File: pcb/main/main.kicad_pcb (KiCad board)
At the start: 2 copper layers, 172.1 x 113 mm, 122 parts, among them J1 Conn_01x04, J10 JTAG, J2 USB_B, J3 Trackball_conn, J4 ROW0, J5 RJ45, J6 ROW1, J7 ROW2, J8 ROW3, J9 STLink, SW1 SW40, SW2 SW41, SW3 SW42, SW4 SW43, SW5 RST_SW, SW6 BOOT0, SW7 BOOT1, U1 3.3v regul, U2 STM32F103C8Tx, Y1 32.768kHz, Y2 8MHz

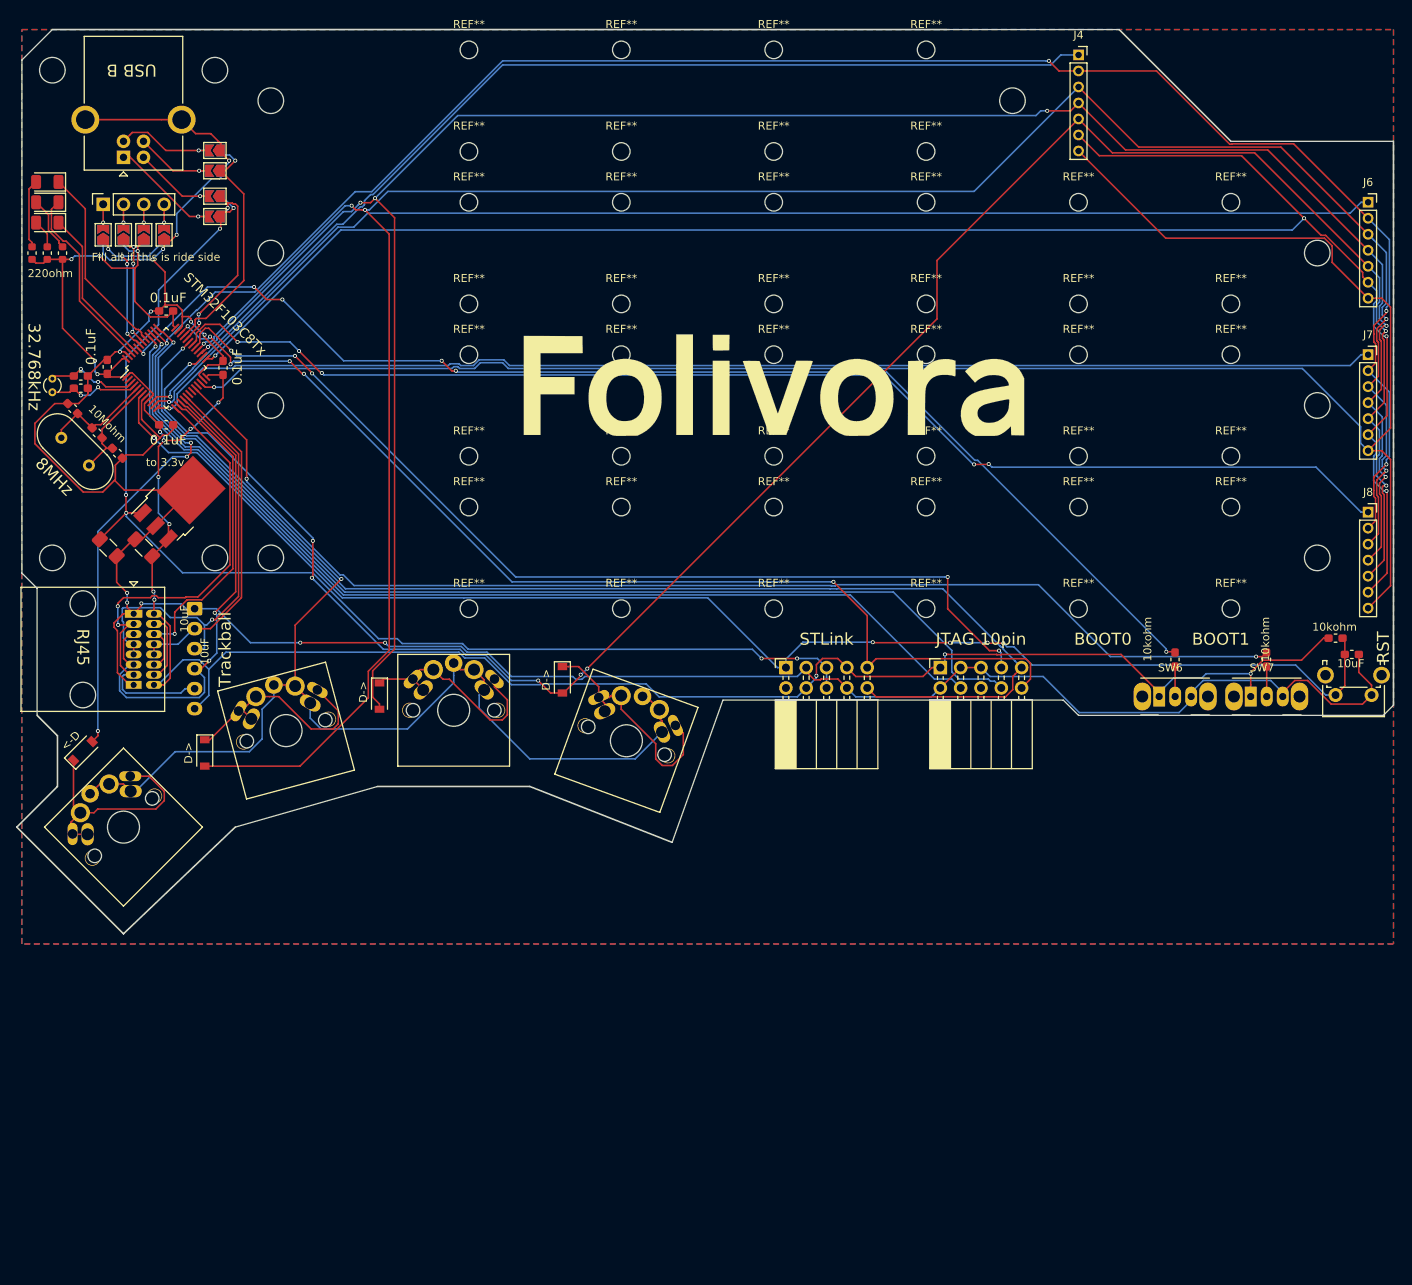
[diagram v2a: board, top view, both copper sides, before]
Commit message: complete pcb design
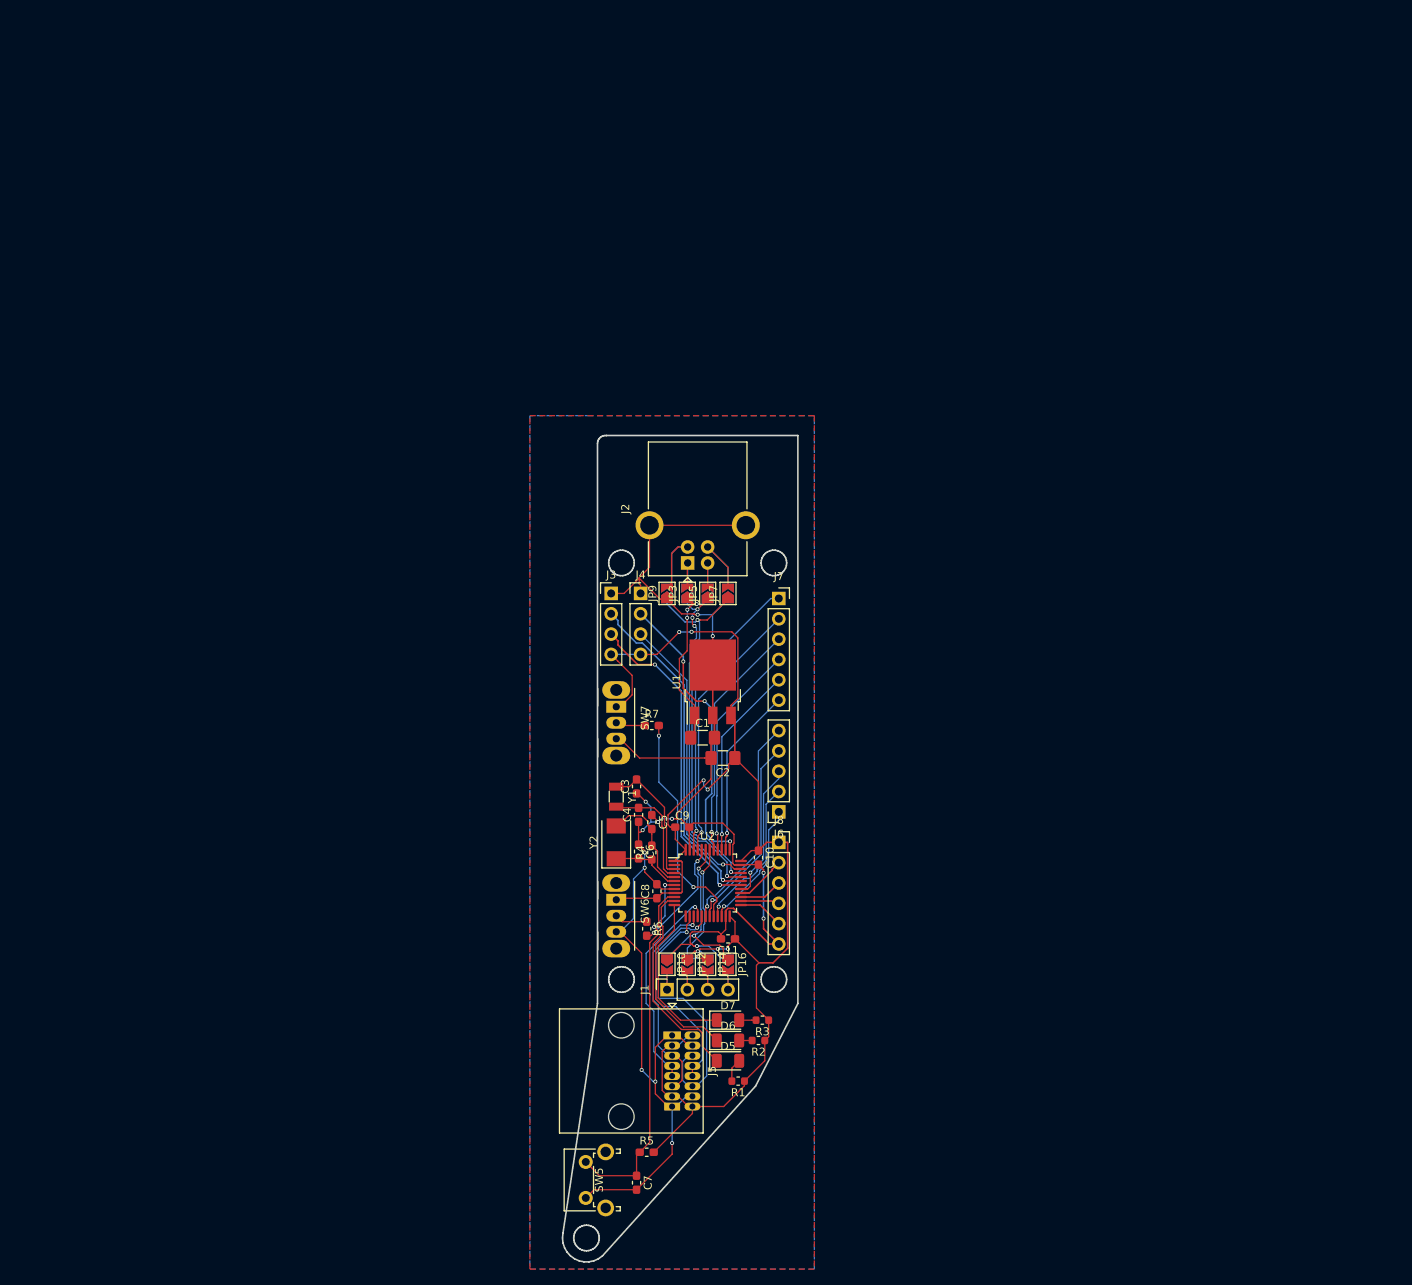
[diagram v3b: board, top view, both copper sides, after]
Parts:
- removed D1, D2, D3, D4: D, Diode_SMD:D_SOD-123
- removed the G*** at (94.0, 44.5) (x2)
- removed J10: JTAG, Connector_PinSocket_2.54mm:PinSocket_2x05_P2.54mm_Horizontal
- removed J9: STLink, Connector_PinSocket_2.54mm:PinSocket_2x05_P2.54mm_Horizontal
- removed REF** (x44): MountingHole_2.2mm_M2, MountingHole:MountingHole_2.2mm_M2
- removed REF** (x12): MountingHole_3.2mm_M3, MountingHole:MountingHole_3.2mm_M3
- removed SW1: SW40, folivora:SW_Cherry_MX1A_1.00u_PCB
- removed SW2: SW41, folivora:SW_Cherry_MX1A_1.00u_PCB
- removed SW3: SW42, folivora:SW_Cherry_MX1A_1.00u_PCB
- removed SW4: SW43, folivora:SW_Cherry_MX1A_1.00u_PCB
- J3: value Trackball_conn -> Serial; footprint Connector_JST:JST_XH_S06B-XH-A_1x06_P2.50mm_Horizontal -> Connector_PinHeader_2.54mm:PinHeader_1x04_P2.54mm_Vertical; moved to F.Cu
- J4: value ROW0 -> STLink; footprint Connector_PinSocket_2.00mm:PinSocket_1x07_P2.00mm_Vertical -> Connector_PinHeader_2.54mm:PinHeader_1x04_P2.54mm_Vertical
- J6: value ROW1 -> SELECT; footprint Connector_PinSocket_2.00mm:PinSocket_1x07_P2.00mm_Vertical -> Connector_PinSocket_2.54mm:PinSocket_1x05_P2.54mm_Vertical
- J7: value ROW2 -> READ; footprint Connector_PinSocket_2.00mm:PinSocket_1x07_P2.00mm_Vertical -> Connector_PinSocket_2.54mm:PinSocket_1x06_P2.54mm_Vertical
- J8: value ROW3 -> TRACKBALL; footprint Connector_PinSocket_2.00mm:PinSocket_1x07_P2.00mm_Vertical -> Connector_PinSocket_2.54mm:PinSocket_1x06_P2.54mm_Vertical
- JP10, JP12, JP14, JP16: moved to F.Cu
- JP11, JP13, JP15, JP17: moved to B.Cu
- Y1: footprint Crystal:Crystal_DS15_D1.5mm_L5.0mm_Vertical -> Crystal:Crystal_SMD_3215-2Pin_3.2x1.5mm
- Y2: footprint Crystal:Crystal_HC49-U_Vertical -> Crystal:Crystal_SMD_Abracon_ABM3-2Pin_5.0x3.2mm
- moved D5 135.0 mm to (88.3, 128.9), turned to 0 degrees
- moved D6 135.0 mm to (88.3, 126.4), turned to 0 degrees
- moved D7 135.0 mm to (88.3, 123.8), turned to 0 degrees
- moved R1 134.8 mm to (89.5, 131.4), turned to 180 degrees
- moved R3 132.4 mm to (92.6, 123.8), turned to 180 degrees
- moved R2 131.4 mm to (92.1, 126.4), turned to 180 degrees
- moved J1 120.9 mm to (80.6, 120.0)
- moved SW5 116.6 mm to (70.5, 146.1), turned to 90 degrees
- moved JP10 115.3 mm to (80.6, 116.8), turned to 270 degrees
- moved JP11 115.3 mm to (80.6, 116.8), turned to 270 degrees
- moved JP12 115.3 mm to (83.2, 116.8), turned to 270 degrees
- moved JP13 115.3 mm to (83.2, 116.8), turned to 270 degrees
- moved JP14 115.3 mm to (85.7, 116.8), turned to 270 degrees
- moved JP15 115.3 mm to (85.7, 116.8), turned to 270 degrees
- moved JP16 115.3 mm to (88.3, 116.8), turned to 270 degrees
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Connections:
- net /SS_K renamed /SS
- J3 pad 2: /MOSI -> /RX
- J3 pad 3: /MISO -> /TX
- J3 pad 4: /SCK -> +3V3
- J4 pad 1: /SELECT0 -> GND
- J4 pad 2: /READ0 -> /SWCLK
- J4 pad 3: /READ1 -> /SWDIO
- J4 pad 4: /READ2 -> +3V3
- J5 pad 2: Net-(J5-Pad2) -> GND
- J5 pad 7: /SS_T -> +3V3
- J6 pad 1: /SELECT1 -> /SELECT0
- J6 pad 2: /READ0 -> /SELECT1
- J6 pad 3: /READ1 -> /SELECT2
- J6 pad 4: /READ2 -> /SELECT3
- J6 pad 5: /READ3 -> /SELECT4
- J7 pad 1: /SELECT2 -> /READ0
- J7 pad 2: /READ0 -> /READ1
- J7 pad 3: /READ1 -> /READ2
- J7 pad 4: /READ2 -> /READ3
- J7 pad 5: /READ3 -> /READ4
- J7 pad 6: /READ4 -> /READ5
- J8 pad 1: /SELECT3 -> +3V3
- J8 pad 2: /READ0 -> /UP
- J8 pad 3: /READ1 -> /DOWN
- J8 pad 4: /READ2 -> /RIGHT
- J8 pad 5: /READ3 -> /LEFT
- J8 pad 6: /READ4 -> GND
- U2 pad 10: /SELECT0 -> /LED1
- U2 pad 11: /SELECT1 -> /LED2
- U2 pad 12: /SELECT2 -> /LED3
- U2 pad 13: /SS_T -> Net-(U2-Pad13)
- U2 pad 18: Net-(U2-Pad18) -> /SELECT4
- U2 pad 19: Net-(U2-Pad19) -> /SELECT3
- U2 pad 21: Net-(U2-Pad21) -> /SELECT1
- U2 pad 22: /READ5 -> /SELECT0
- U2 pad 25: /READ4 -> /LEFT
- U2 pad 26: /READ3 -> /RIGHT
- U2 pad 27: /READ2 -> /DOWN
- U2 pad 28: /READ1 -> /UP
- U2 pad 29: /JTDI -> /SELECT2
- U2 pad 30: /SELECT3 -> /TX
- U2 pad 31: /SELECT4 -> /RX
- U2 pad 38: /READ0 -> /READ5
- U2 pad 39: /JTDO -> /READ4
- U2 pad 40: /JNTRST -> /READ3
- U2 pad 41: /LED3 -> /READ2
- U2 pad 45: /LED1 -> /READ1
- U2 pad 46: /LED2 -> /READ0
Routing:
- net /READ1: track 299.2 -> 33.4 mm, vias 5 -> 1
- net /READ2: track 276.7 -> 29.9 mm, vias 6 -> 1
- net /READ0: track 277.8 -> 36.5 mm, vias 7 -> 1
- net /READ3: track 262.7 -> 27.0 mm, vias 8 -> 1
- net /READ5: track 243.8 -> 21.4 mm
- net /READ4: track 232.3 -> 24.2 mm, vias 4 -> 1
- net /SELECT1: track 163.0 -> 19.2 mm
- net /BOOT0: track 152.9 -> 14.2 mm, vias 6 -> 2
- net /SELECT2: track 155.7 -> 17.2 mm
- net /SELECT4: track 161.4 -> 27.3 mm, vias 2 -> 1
- net /SELECT3: track 158.4 -> 24.5 mm, vias 5 -> 1
- net /JTDO: track 132.9 -> 0.00 mm, vias 1 -> 0
- net /RST: track 178.5 -> 46.4 mm, vias 5 -> 2
- net +5V: track 151.3 -> 21.9 mm, vias 6 -> 3
- net /JNTRST: track 126.0 -> 0.00 mm, vias 1 -> 0
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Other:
- board size 172.1 x 113 mm -> 29.4 x 103.3 mm
- board text removed: "0.1uF"
- board text removed: "10Mohm"
- board text removed: "10kohm"
- board text removed: "10uF"
- board text removed: "220ohm"
- board text removed: "32.768kHz"
- board text removed: "8MHz"
- board text removed: "<-D"
- board text removed: "BOOT0"
- board text removed: "BOOT1"
- board text removed: "D->"
- board text removed: "Fill all if this is ride side"
- board text removed: "JTAG 10pin"
- board text removed: "RJ45"
- board text removed: "RST"
- board text removed: "STLink"
- board text removed: "STM32F103C8Tx"
- board text removed: "Trackball"
- board text removed: "USB B"
- board text removed: "to 3.3v"
